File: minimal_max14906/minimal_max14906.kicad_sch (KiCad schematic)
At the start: 117 parts, among them J10 TBP02R2-381-02BE, J11 TBP02R2-381-02BE, J12 CLP-102-02-G-D-BE, J13 CLP-108-02-G-D-BE, J14 CLP-108-02-G-D-BE, J15 CLP-102-02-G-D-BE, J2 TBP02R2-381-02BE, J3 TBP02R2-381-02BE, J4 CLP-102-02-G-D-BE, J5 CLP-102-02-G-D-BE, J6 CLP-102-02-G-D-BE, J7 CLP-102-02-G-D-BE, J8 CLP-102-02-G-D-BE, Q1 -60.0 V, Q2 -60.0 V, Q3 -60.0 V, Q4 -60.0 V, Q5 100 V, Q6 100 V, U1 ADUM1252AUA+, U2 MAX22441CAEE+, U3 MAX22442CAEE+, U4 ADUM1252AUA+, U5 MAX14906ATM+, U6 ADUM1252AUA+

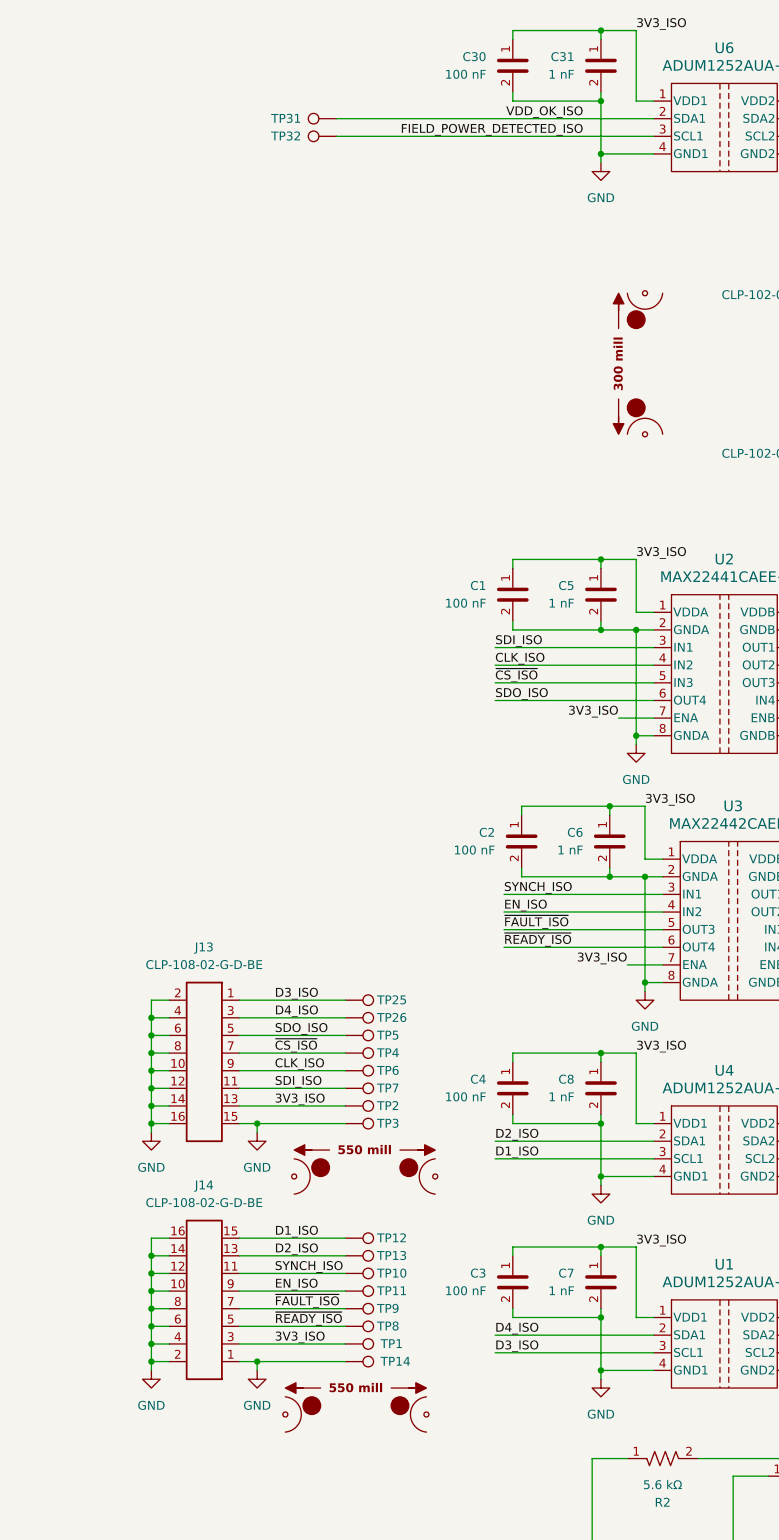
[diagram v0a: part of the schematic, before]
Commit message: development backup
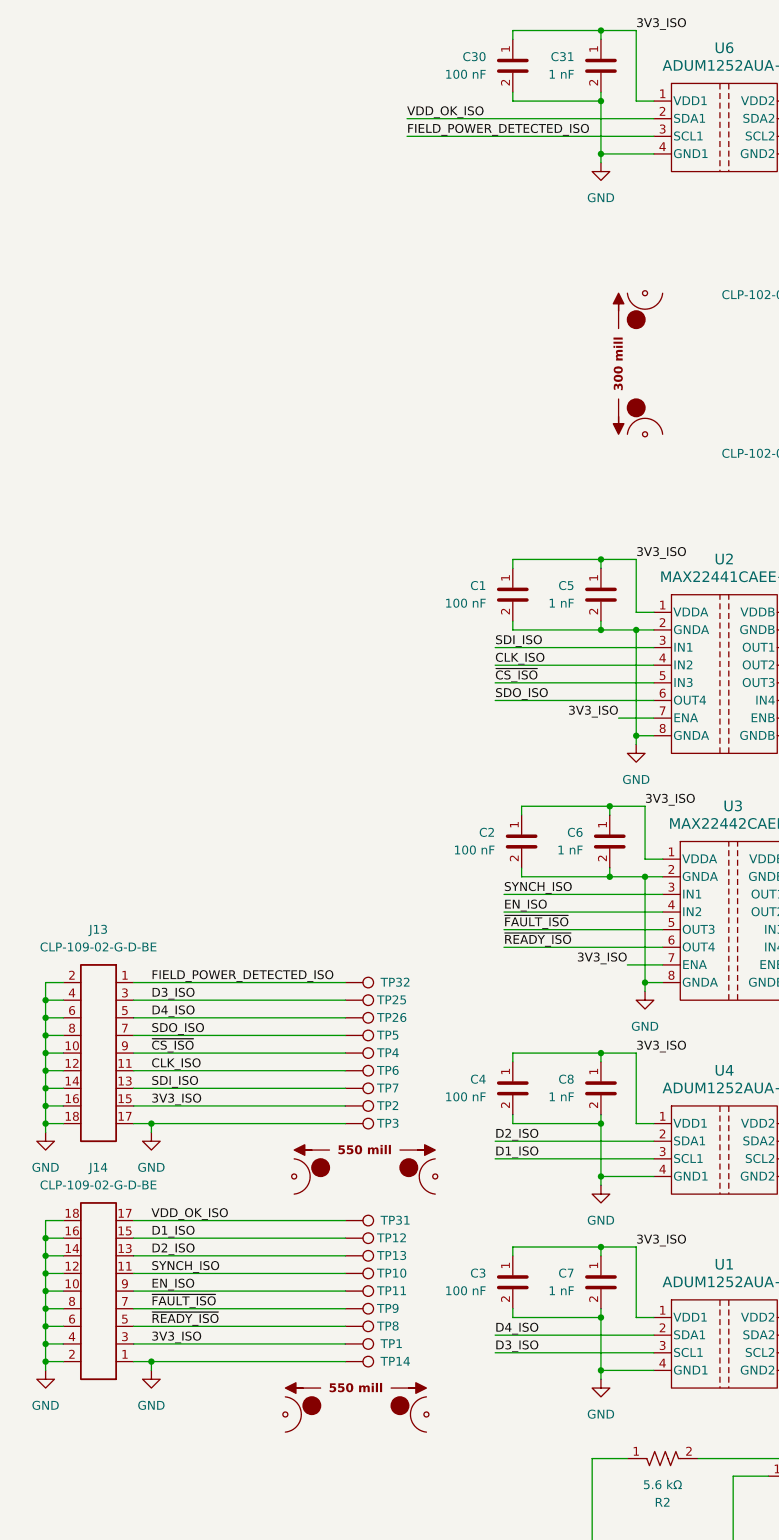
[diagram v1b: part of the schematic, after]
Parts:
- J13, J14: value CLP-108-02-G-D-BE -> CLP-109-02-G-D-BE; footprint connector_footprints:CLP-108-02-G-D-BE -> connector_footprints:CLP-109-02-G-D-BE; symbol UNITED_CONNECTORS_DATA_BASE:J_CLP-108-02-G-D-BE -> UNITED_CONNECTORS_DATA_BASE:J_CLP-109-02-G-D-BE; MPN CLP-108-02-G-D-BE -> CLP-109-02-G-D-BE; Pin Count 8 -> 9; Symbol Name J_CLP-108-02-G-D-BE -> J_CLP-109-02-G-D-BE; Trustedparts Search https://www.trustedparts.com/en/search/CLP-108-02-G-D-BE -> https://www.trustedparts.com/en/search/CLP-109-02-G-D-BE
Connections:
- net 3V3_ISO: now also J13.15; no longer J13.13
- net CLK_ISO: now also J13.11; no longer J13.9
- net D3_ISO: now also J13.3; no longer J13.1
- net D4_ISO: now also J13.5; no longer J13.3
- net FIELD_POWER_DETECTED_ISO: now also J13.1
- net GND: now also J13.17, J13.18, J14.18; no longer J13.15
- net SDI_ISO: now also J13.13; no longer J13.11
- net SDO_ISO: now also J13.7; no longer J13.5
- net VDD_OK_ISO: now also J14.17
- net ~{CS_ISO}: now also J13.9; no longer J13.7
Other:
- moved on the sheet: TP31, TP32
